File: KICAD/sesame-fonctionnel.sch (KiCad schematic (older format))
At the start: 9 parts

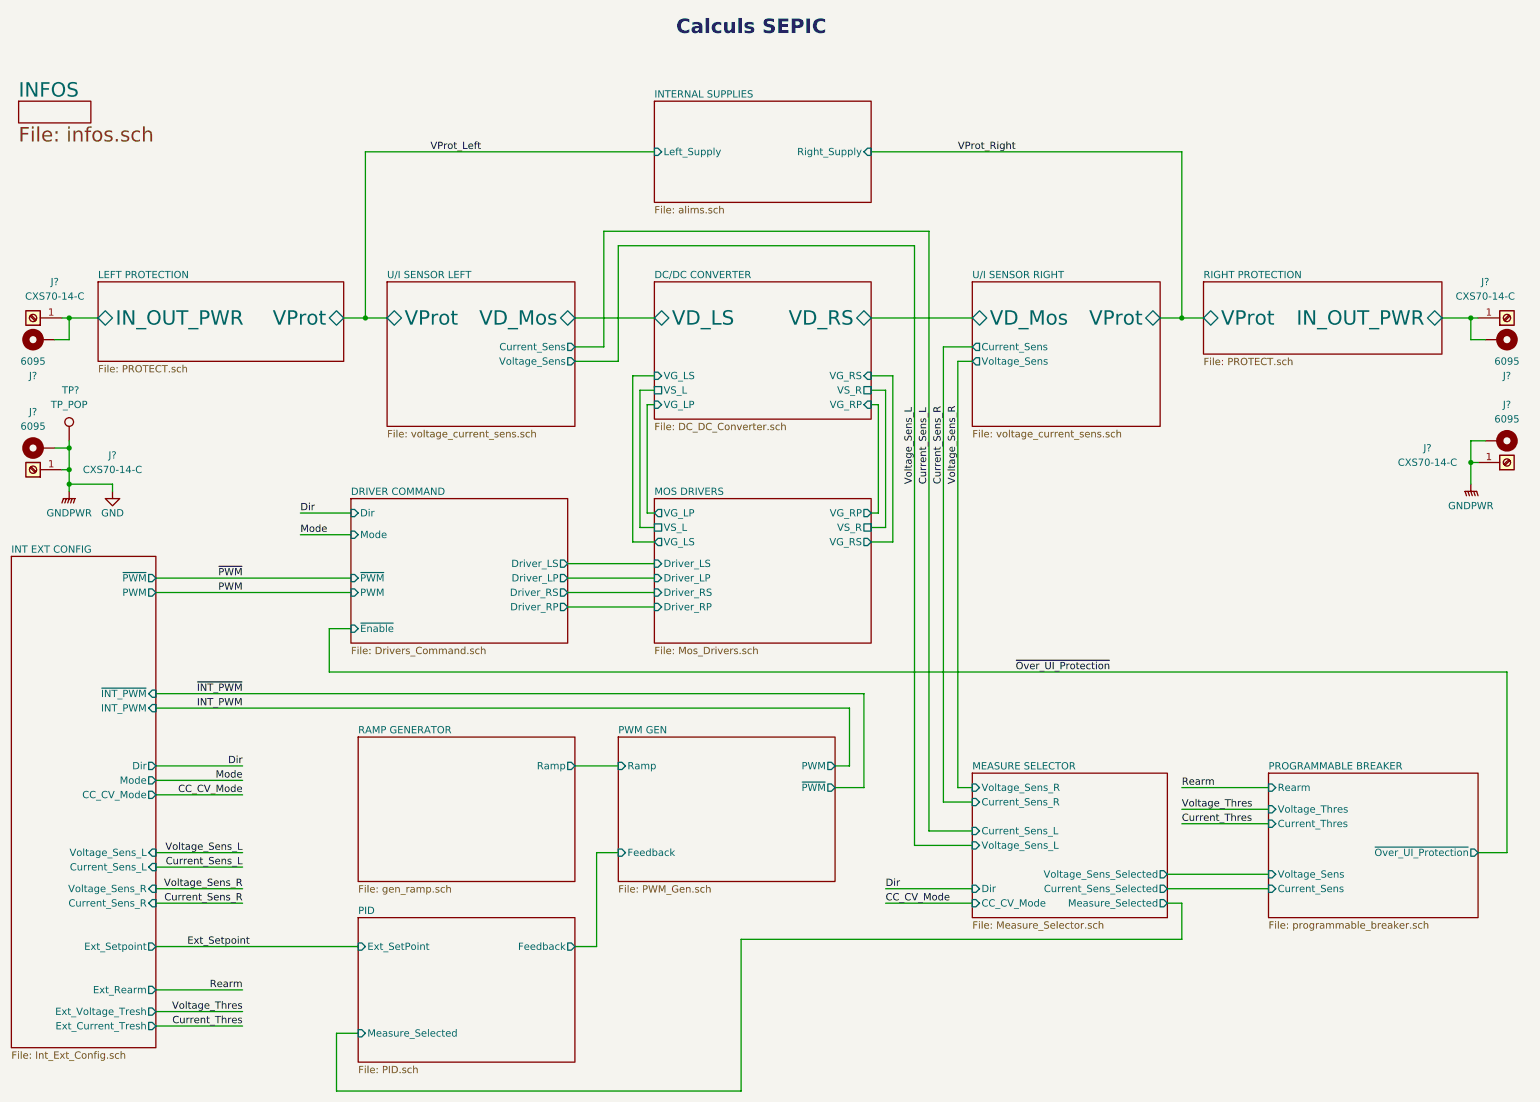
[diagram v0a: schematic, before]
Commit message: driver + clean clean clean
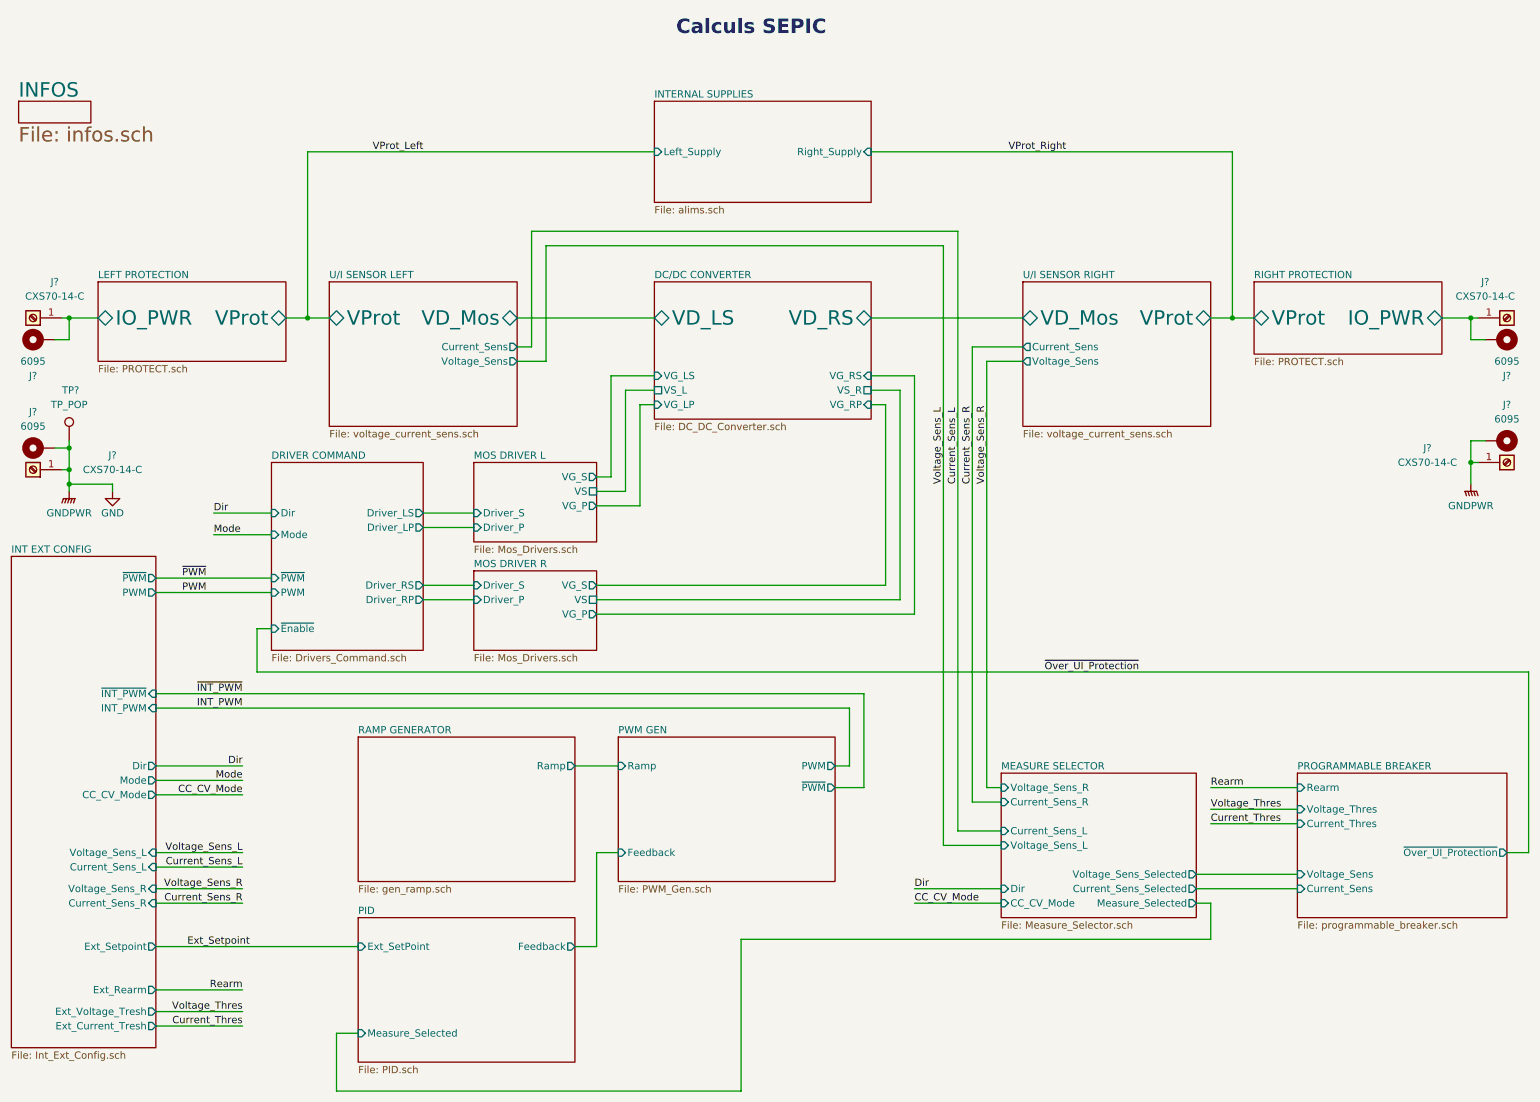
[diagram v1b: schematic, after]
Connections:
- net LEFT PROTECTION/IN_OUT_PWR renamed LEFT PROTECTION/IO_PWR
- net RIGHT PROTECTION/IN_OUT_PWR renamed RIGHT PROTECTION/IO_PWR
